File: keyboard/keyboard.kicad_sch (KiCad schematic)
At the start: 52 parts, among them J2 USB2.0, U1 BQ24075RGT, U3 nRF52840, U7 ESDR0502NMUTAG, Y1 32MHz, Y2 32.768 kHz

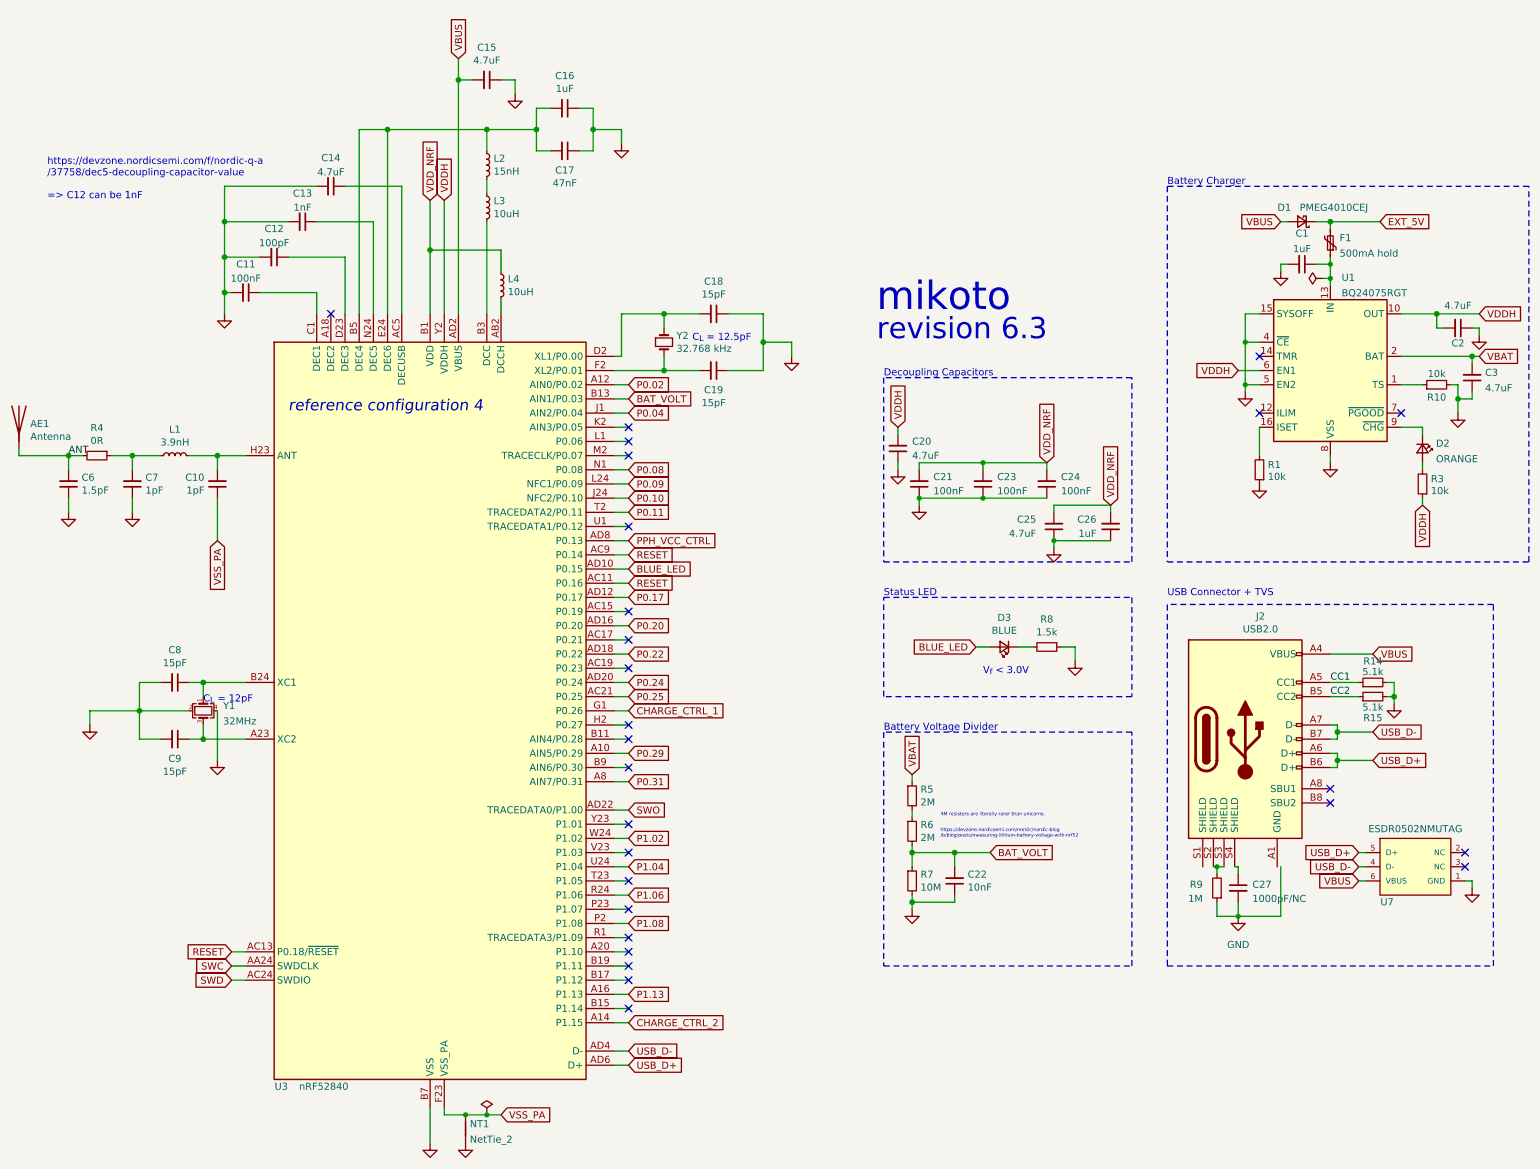
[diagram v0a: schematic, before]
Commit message: keyboard v1 halfway routed
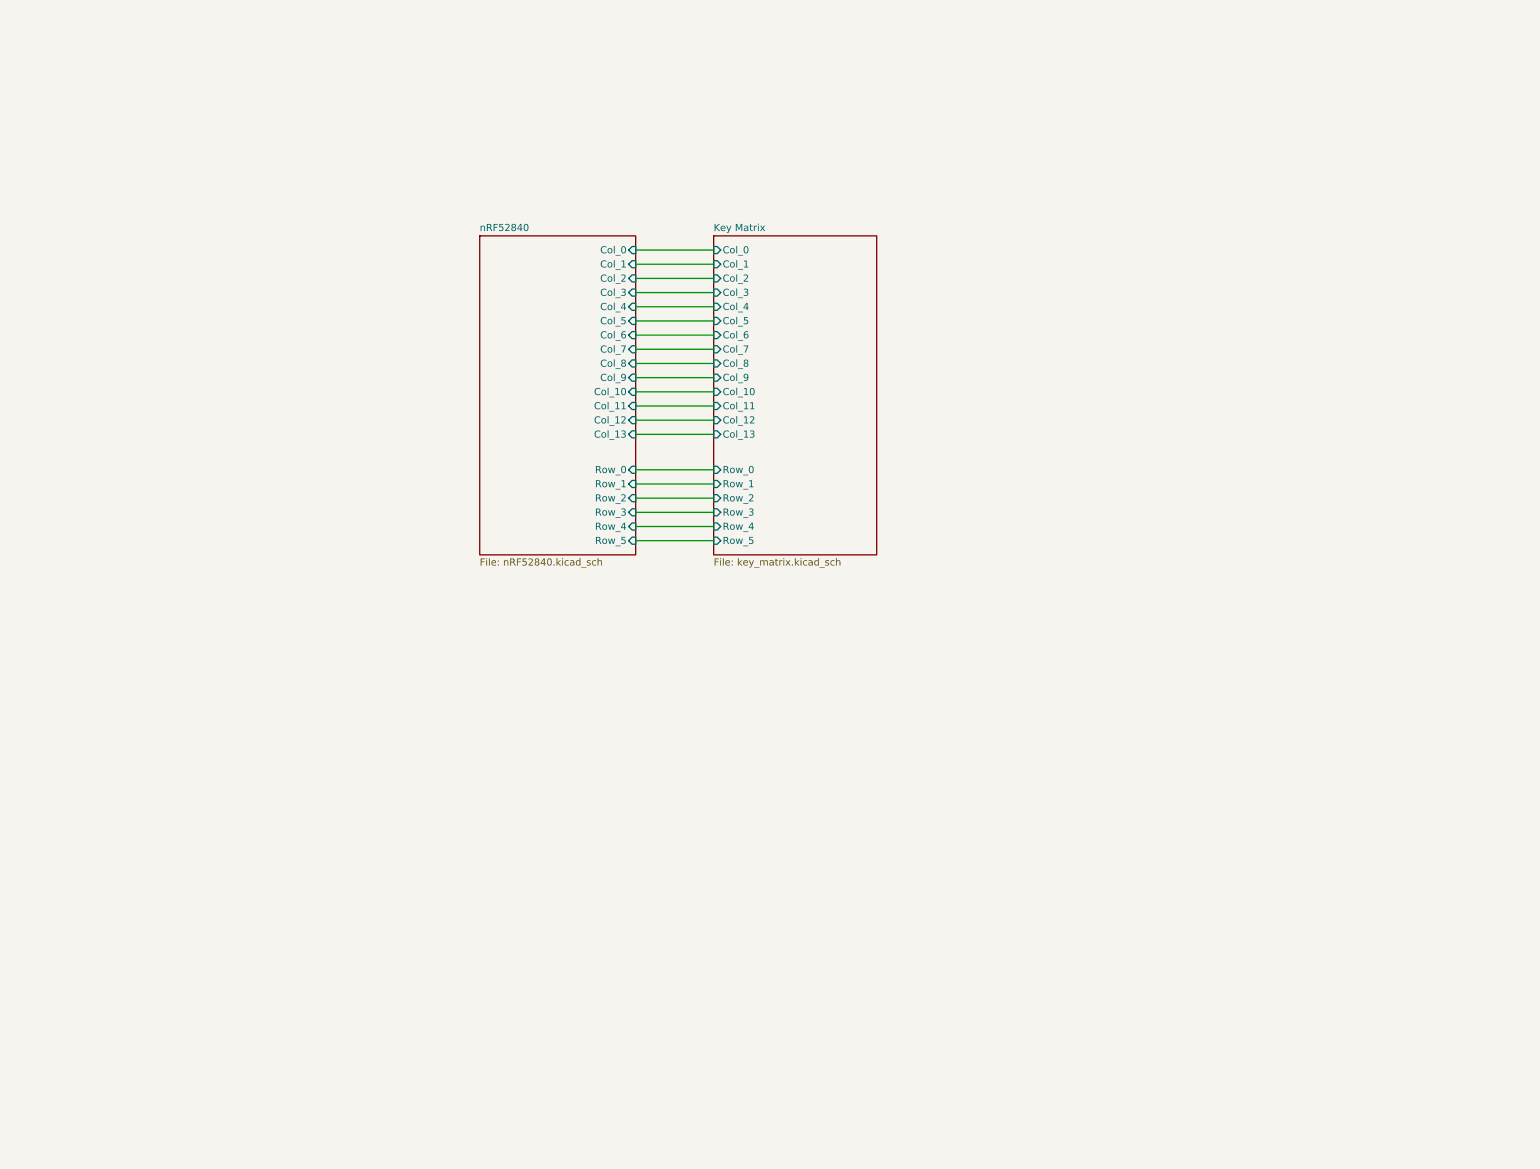
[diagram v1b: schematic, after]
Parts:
- removed AE1: Antenna, footprints:2.4GHz-meander-antenna-v2, symbol Device:Antenna
- removed C1, C16, C26: 1uF, footprints:Capacitor_0402_1005M-nosilk, symbol Device:C_Small
- removed C10, C7: 1pF, footprints:Capacitor_0402_1005M-nosilk, symbol Device:C_Small
- removed C11, C21, C23, C24: 100nF, footprints:Capacitor_0402_1005M-nosilk, symbol Device:C_Small
- removed C12: 100pF, footprints:Capacitor_0402_1005M-nosilk, symbol Device:C_Small
- removed C13: 1nF, footprints:Capacitor_0402_1005M-nosilk, symbol Device:C_Small
- removed C14, C15, C2, C20, C25, C3: 4.7uF, footprints:Capacitor_0402_1005M-nosilk, symbol Device:C_Small
- removed C17: 47nF, footprints:Capacitor_0402_1005M-nosilk, symbol Device:C_Small
- removed C18, C19, C8, C9: 15pF, footprints:Capacitor_0402_1005M-nosilk, symbol Device:C_Small
- removed C22: 10nF, footprints:Capacitor_0402_1005M-nosilk, symbol Device:C_Small
- removed C27: 1000pF/NC, Capacitor_SMD:C_0402_1005Metric, symbol Device:C_Small
- removed C6: 1.5pF, footprints:Capacitor_0402_1005M-nosilk, symbol Device:C_Small
- removed D1: PMEG4010CEJ, footprints:D_SOD-323F-nosilk, symbol Device:D_Schottky_Small
- removed D2: ORANGE, footprints:LED_0603_1608Metric-nosilk, symbol Device:LED_Small
- removed D3: BLUE, footprints:LED_0603_1608Metric-nosilk, symbol Device:LED_Small
- removed F1: 500mA hold, footprints:Fuse_0402_1005Metric, symbol Device:Polyfuse_Small
- removed J2: USB2.0, footprints:USB-C_C168688, symbol mikoto:USB_C_Receptacle_USB2.0
- removed L1: 3.9nH, footprints:Inductor_0402_1005M-nosilk, symbol Device:L_Small
- removed L2: 15nH, footprints:Inductor_0402_1005M-nosilk, symbol Device:L_Small
- removed L3, L4: 10uH, footprints:Inductor_0603_1608M-nosilk, symbol Device:L_Small
- removed NT1: NetTie_2, footprints:net-tie-2-tiny, symbol Device:NetTie_2
- removed R1, R10, R3: 10k, footprints:Resistor_0402_1005M-nosilk, symbol Device:R_Small
- removed R14, R15: 5.1k, footprints:Resistor_0402_1005M-nosilk, symbol Device:R_Small
- removed R4: 0R, footprints:Resistor_0402_1005M-nosilk, symbol Device:R_Small
- removed R5, R6: 2M, footprints:Resistor_0402_1005M-nosilk, symbol Device:R_Small
- removed R7: 10M, footprints:Resistor_0402_1005M-nosilk, symbol Device:R_Small
- removed R8: 1.5k, footprints:Resistor_0402_1005M-nosilk, symbol Device:R_Small
- removed R9: 1M, Resistor_SMD:R_0402_1005Metric, symbol Device:R_Small
- removed U1: BQ24075RGT, footprints:VQFN-16-1EP_3x3mm_P0.5mm_EP1.6x1.6mm, symbol Battery_Management:BQ24075RGT
- removed U3: nRF52840, footprints:AQFN-73-1EP_7x7mm_P0.5mm_NRF52840-custom, symbol MCU_Nordic:nRF52840
- removed U7: ESDR0502NMUTAG, footprints:UDFN-6_1.2x1.0mm_P0.4mm, symbol mikoto:ESDR0502NMUTAG
- removed Y1: 32MHz, footprints:Crystal_SMD_2016-4Pin_2.0x1.6mm, symbol Device:Crystal_GND24_Small
- removed Y2: 32.768 kHz, footprints:Crystal_SMD_2012-2Pin_2.0x1.2mm, symbol Device:Crystal_Small
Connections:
- no-connect marks 27 -> 0
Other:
- added sheet Key Matrix (key_matrix.kicad_sch)
- added sheet nRF52840 (nRF52840.kicad_sch)
- note removed: "4M resistors are literally rarer than unicorns."
- note removed: "Battery Charger"
- note removed: "Battery Voltage Divider"
- note removed: "C_{L} = 12.5pF"
- note removed: "C_{L} = 12pF"
- note removed: "Decoupling Capacitors"
- note removed: "Status LED"
- note removed: "USB Connector + TVS"
- note removed: "V_{f} < 3.0V"
- note removed: "https://devzone.nordicsemi.com/f/nordic-q-a /37758/dec5-decoupling-capacitor-value => C12 can be 1nF"
- note removed: "https://devzone.nordicsemi.com/nordic/nordic-blog /b/blog/posts/measuring-lithium-battery-voltage-with-nrf52"
- note removed: "mikoto"
- note removed: "reference configuration 4"
- note removed: "revision 6.3"
- company: (none) -> Byran Technologies
- title: (none) -> Laptop Keyboard
